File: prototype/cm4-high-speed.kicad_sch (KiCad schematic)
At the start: 10 parts, among them J2 54548-2271, J3 USB4105-GF-A, U2 TPD2EUSB30

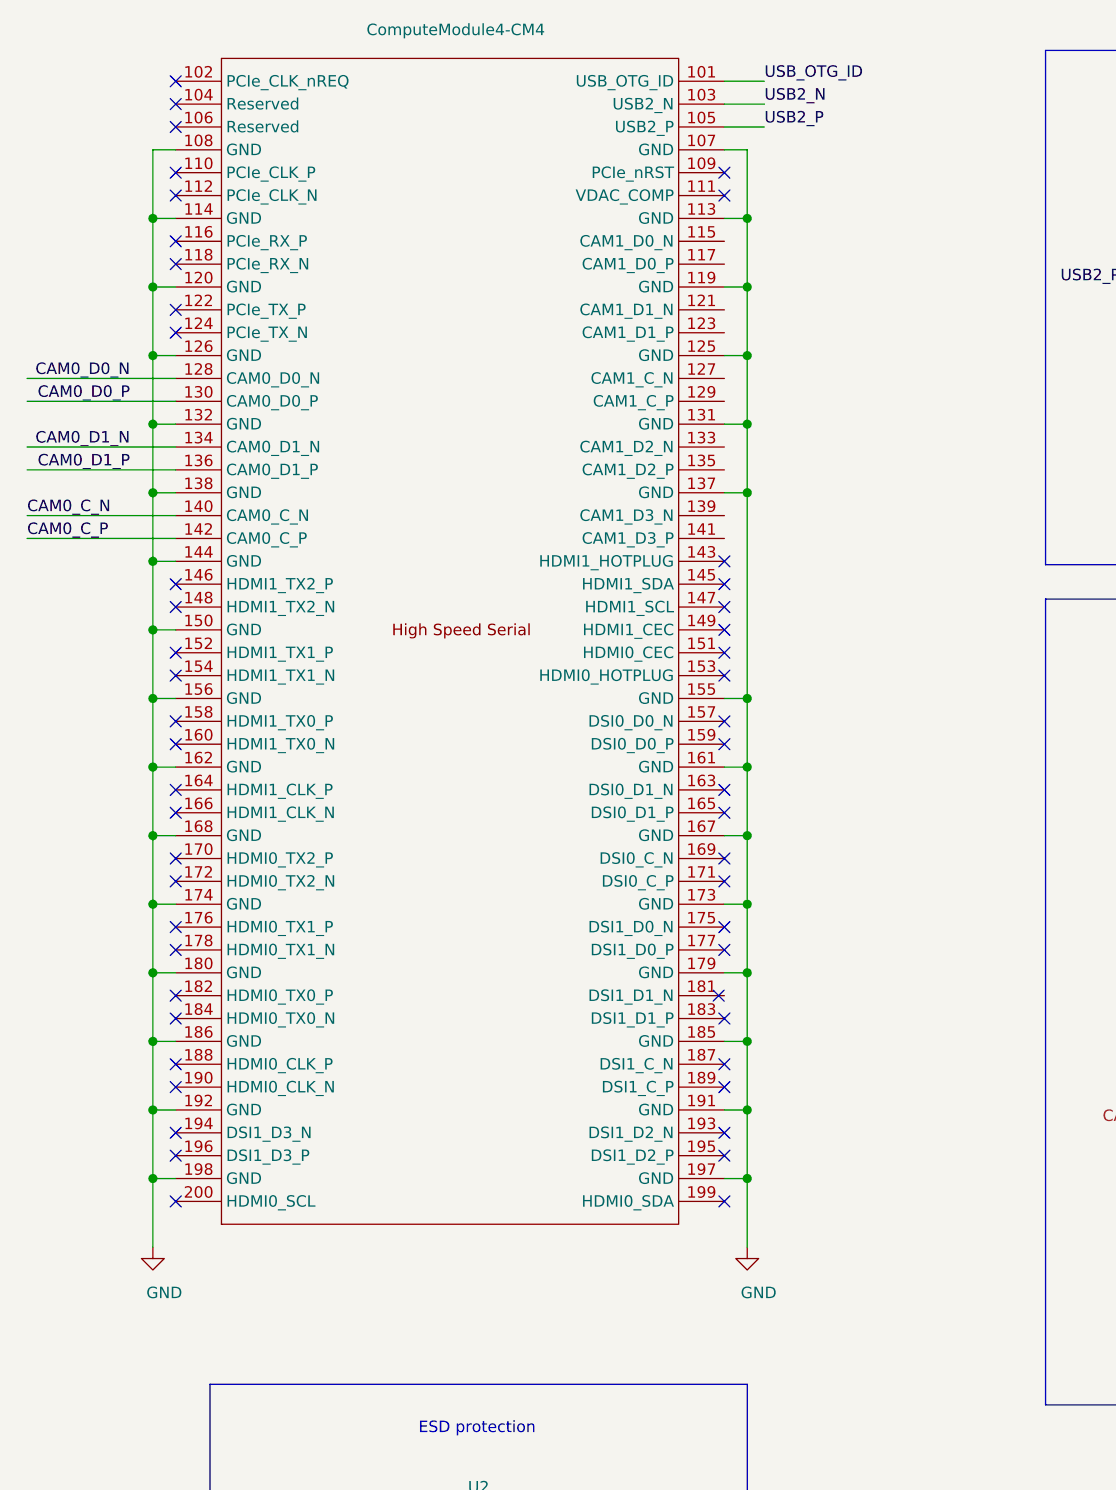
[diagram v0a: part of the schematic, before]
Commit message: -
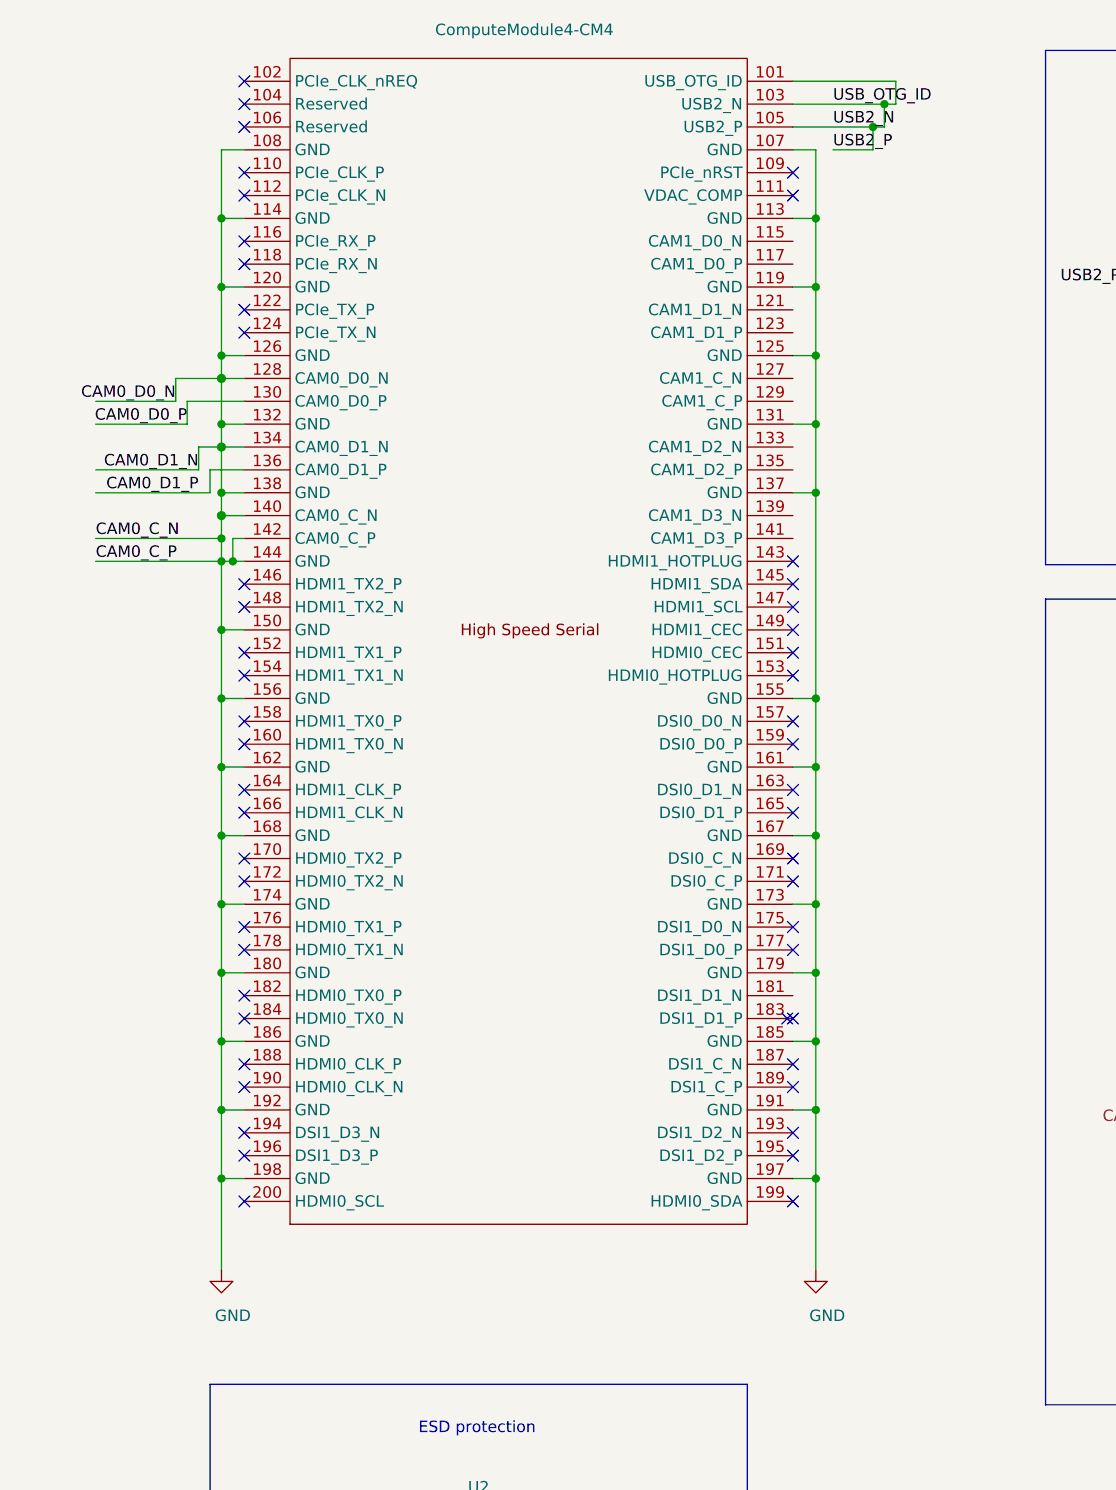
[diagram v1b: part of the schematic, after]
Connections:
- net CAM0_C_N is gone; now on net GND: J2.8, Module1.140 (CAM0_C_N)
- net CAM0_C_P is gone; now on net GND: J2.9, Module1.142 (CAM0_C_P)
- net CAM0_D0_N is gone; now on net GND: J2.2, Module1.128 (CAM0_D0_N)
- net CAM0_D1_N is gone; now on net GND: J2.5, Module1.134 (CAM0_D1_N)
- net USB2_P is gone; now on net USB2_N: J3.A6 (DP1), J3.B6 (DP2), Module1.105 (USB2_P), U2.1 (D+)
- net USB_OTG_ID is gone; now on net USB2_N: Module1.101 (USB_OTG_ID), R11.2, R12.1
